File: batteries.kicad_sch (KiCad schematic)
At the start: 2 parts, among them U11 TCA9546AD

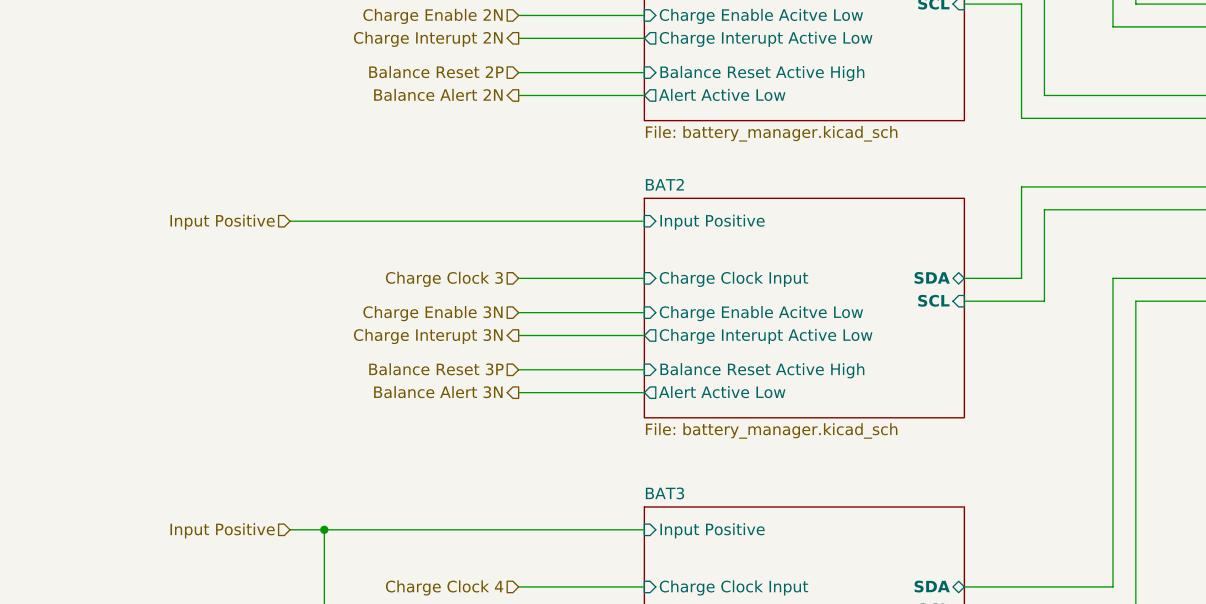
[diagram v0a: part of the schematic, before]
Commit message: not adding this to source control months ago was one of the dumbest things i've ever done. and im not particularly risk-avers
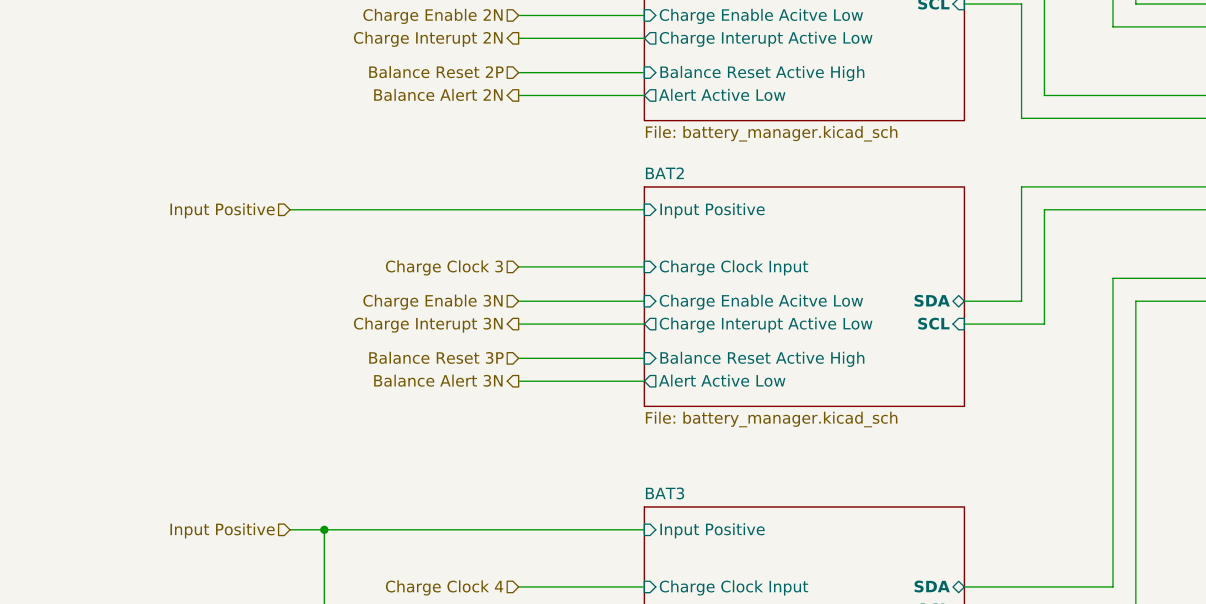
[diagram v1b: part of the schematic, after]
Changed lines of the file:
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@@
 	(wire
 		(pts
-			(xy 170.18 115.57) (xy 170.18 105.41)
+			(xy 170.18 118.11) (xy 170.18 105.41)
 		)
 		(stroke
@@
 	(wire
 		(pts
-			(xy 163.83 115.57) (xy 170.18 115.57)
-		)
-		(stroke
-			(width 0)
-			(type default)
-		)
-	)
-	(wire
-		(pts
-			(xy 114.3 128.27) (xy 128.27 128.27)
+			(xy 163.83 118.11) (xy 170.18 118.11)
+		)
+		(stroke
+			(width 0)
+			(type default)
+		)
+	)
+	(wire
+		(pts
+			(xy 114.3 127) (xy 128.27 127)
 		)
 		(stroke
@@
 	(wire
 		(pts
-			(xy 114.3 115.57) (xy 128.27 115.57)
+			(xy 114.3 114.3) (xy 128.27 114.3)
 		)
 		(stroke
@@
 	(wire
 		(pts
-			(xy 88.9 109.22) (xy 128.27 109.22)
+			(xy 88.9 107.95) (xy 128.27 107.95)
 		)
 		(stroke
@@
 	(wire
 		(pts
-			(xy 114.3 119.38) (xy 128.27 119.38)
+			(xy 114.3 118.11) (xy 128.27 118.11)
 		)
 		(stroke
@@
 	(wire
 		(pts
-			(xy 114.3 121.92) (xy 128.27 121.92)
+			(xy 114.3 120.65) (xy 128.27 120.65)
 		)
 		(stroke
@@
 	(wire
 		(pts
-			(xy 163.83 118.11) (xy 172.72 118.11)
+			(xy 163.83 120.65) (xy 172.72 120.65)
 		)
 		(stroke
@@
 	(wire
 		(pts
-			(xy 172.72 118.11) (xy 172.72 107.95)
+			(xy 172.72 120.65) (xy 172.72 107.95)
 		)
 		(stroke
@@
 	(wire
 		(pts
-			(xy 114.3 125.73) (xy 128.27 125.73)
+			(xy 114.3 124.46) (xy 128.27 124.46)
 		)
 		(stroke
@@
 	(hierarchical_label "Balance Reset 3P"
 		(shape input)
-		(at 114.3 125.73 180)
+		(at 114.3 124.46 180)
 		(effects
 			(font
@@
 	(hierarchical_label "Charge Clock 3"
 		(shape input)
-		(at 114.3 115.57 180)
+		(at 114.3 114.3 180)
 		(effects
 			(font
@@
 	(hierarchical_label "Charge Interupt 3N"
 		(shape output)
-		(at 114.3 121.92 180)
+		(at 114.3 120.65 180)
 		(effects
 			(font
@@
 	(hierarchical_label "Balance Alert 3N"
 		(shape output)
-		(at 114.3 128.27 180)
+		(at 114.3 127 180)
 		(effects
 			(font
@@
 	(hierarchical_label "Input Positive"
 		(shape input)
-		(at 88.9 109.22 180)
+		(at 88.9 107.95 180)
 		(effects
 			(font
@@
 	(hierarchical_label "Charge Enable 3N"
 		(shape input)
-		(at 114.3 119.38 180)
+		(at 114.3 118.11 180)
 		(effects
 			(font
@@
 	)
 	(sheet
-		(at 128.27 106.68)
+		(at 128.27 105.41)
 		(size 35.56 24.384)
 		(exclude_from_sim no)
@@
 		)
 		(property "Sheetname" "BAT2"
-			(at 128.27 105.9684 0)
+			(at 128.27 104.6984 0)
 			(effects
 				(font
@@
 		)
 		(property "Sheetfile" "battery_manager.kicad_sch"
-			(at 128.27 131.6486 0)
+			(at 128.27 130.3786 0)
 			(effects
 				(font
@@
 		)
 		(pin "Alert Active Low" output
-			(at 128.27 128.27 180)
+			(at 128.27 127 180)
 			(effects
 				(font
@@
 		)
 		(pin "Balance Reset Active High" input
-			(at 128.27 125.73 180)
+			(at 128.27 124.46 180)
 			(effects
 				(font
@@
 		)
 		(pin "Charge Clock Input" input
-			(at 128.27 115.57 180)
+			(at 128.27 114.3 180)
 			(effects
 				(font
@@
 		)
 		(pin "Charge Enable Acitve Low" input
-			(at 128.27 119.38 180)
+			(at 128.27 118.11 180)
 			(effects
 				(font
@@
 		)
 		(pin "Charge Interupt Active Low" output
-			(at 128.27 121.92 180)
+			(at 128.27 120.65 180)
 			(effects
 				(font
@@
 		)
 		(pin "SCL" input
-			(at 163.83 118.11 0)
+			(at 163.83 120.65 0)
 			(effects
 				(font
@@
 		)
 		(pin "SDA" bidirectional
-			(at 163.83 115.57 0)
+			(at 163.83 118.11 0)
 			(effects
 				(font
@@
 		)
 		(pin "Input Positive" input
-			(at 128.27 109.22 180)
-			(effects
-				(font
+			(at 128.27 107.95 180)
+			(effects
+				(font
